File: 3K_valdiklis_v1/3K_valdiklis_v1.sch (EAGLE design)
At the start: 67 parts, among them IC2 L293D, IC4 ATMEGA1284, IC5 DS1307, J4 HEAD3X2, K1 S202T02, K2 S202T02, K3 S202T02, K4 S202T02, K5 S202T02, K6 S202T02, Q4 32.768, T2 TIP120V, X1 Boiler pump, X10 22-23-2031, X11 +12V, X2 Storage tank pump, X3 Radiator pump, X4 4 way valve 1, X5 4 way valve 2, X6 Floor heating, X7 motorized valve 1, X77 PUMP1, X8 motorized valve 2, X9 16MHz, Y1 12mhz

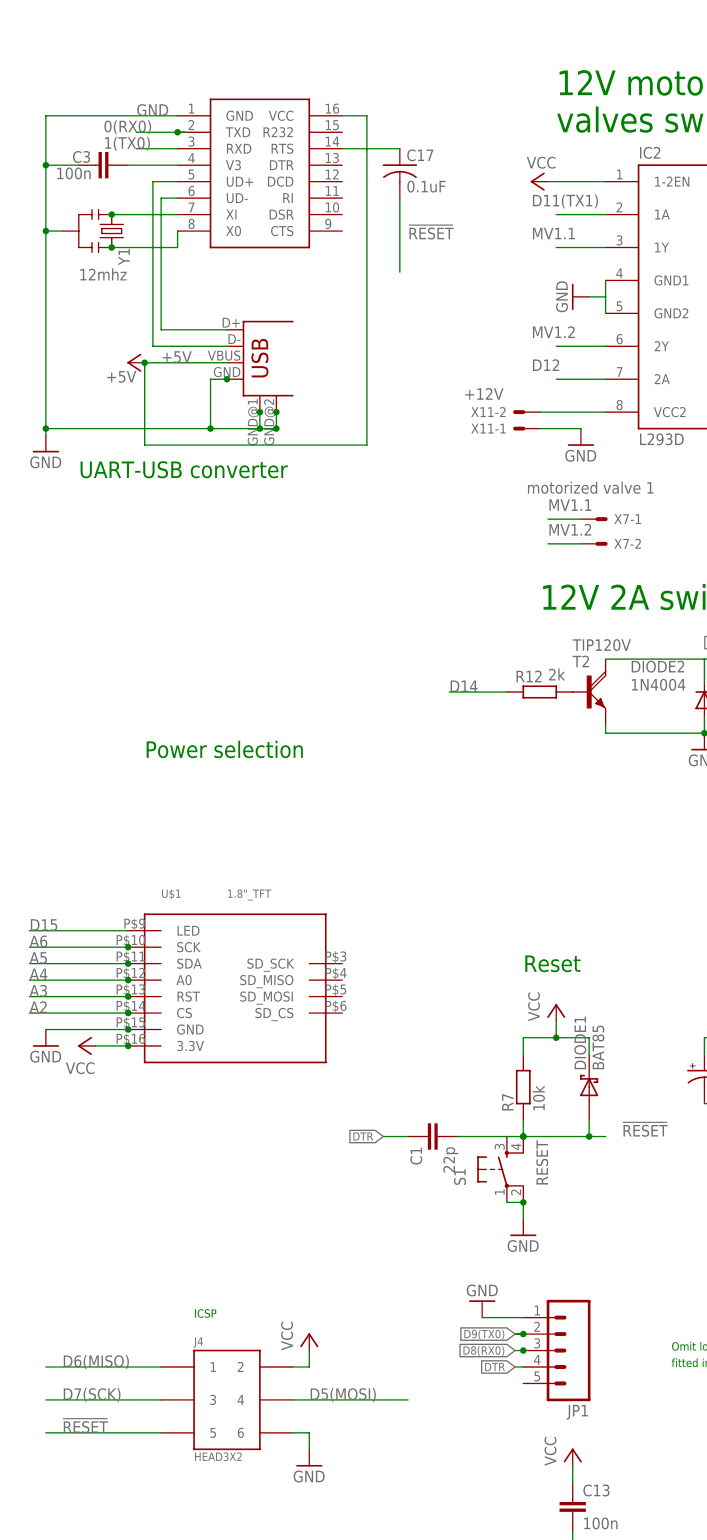
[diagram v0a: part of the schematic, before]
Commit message: trasavimas
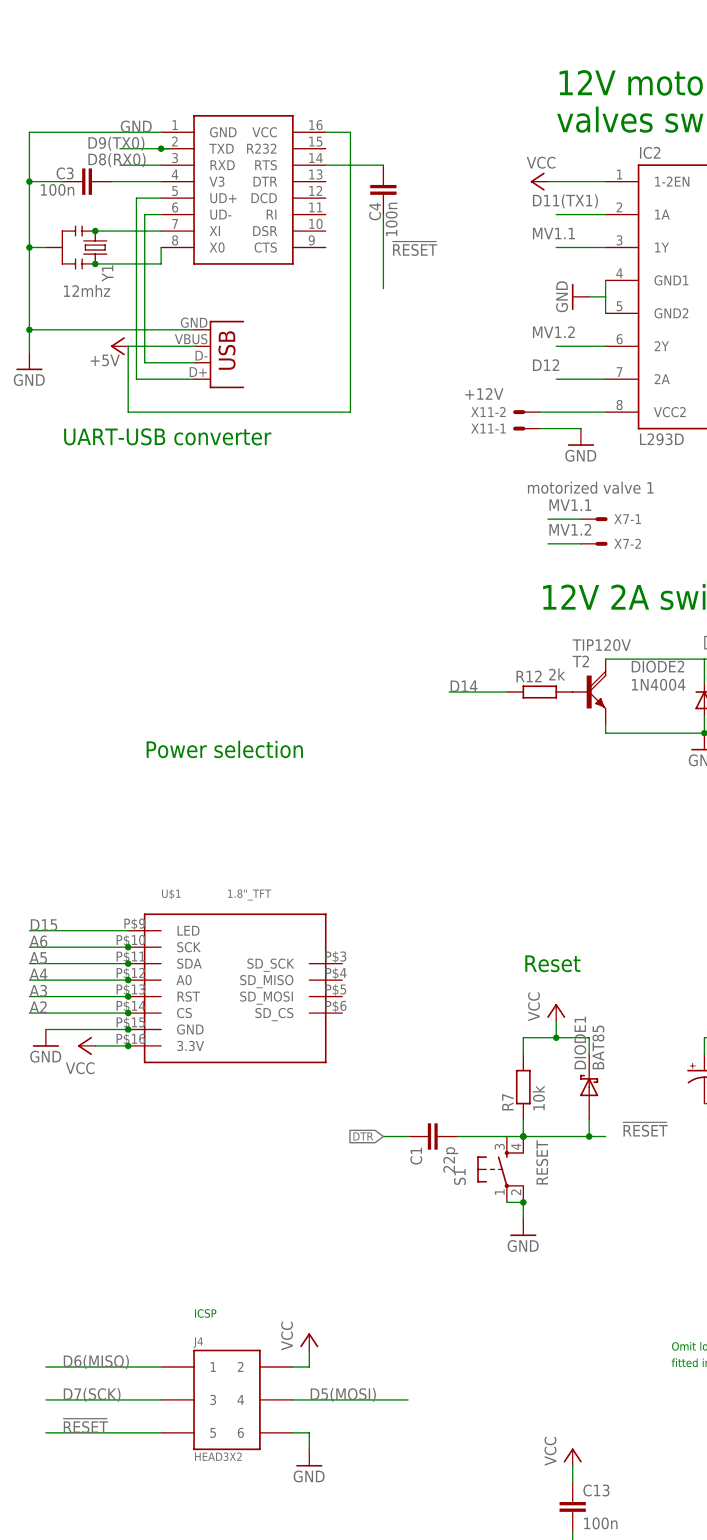
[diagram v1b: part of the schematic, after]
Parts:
- removed C17: 0.1uF, rcl:C-USC0805K
- removed JP1: (no value), SparkFun-Connectors-1:M05PTH
- removed USB1: USB-B-H, con-usb-2:USB-B-H
- added C4: 100n, SparkFun:CAPPTH
- added JP3: USB-B, SparkFun-Connectors-1:USBPTH
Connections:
- removed net 0(RX0): U$2.TXD
- removed net 1(TX0): U$2.RXD
- net !RESET: now also C4.1; no longer C17.2
- net +5V: now also JP3.VBUS; no longer USB1.VBUS
- net D8(RX0): now also U$2.RXD; no longer JP1.3
- net D9(TX0): now also U$2.TXD; no longer JP1.2
- net DTR: no longer JP1.4
- net GND: now also JP3.GND; no longer JP1.1, USB1.GND, USB1.GND@1, USB1.GND@2
- net N$11: now also C4.2; no longer C17.1
- net N$12: now also JP3.D-; no longer USB1.D+
- net N$22: now also JP3.D+; no longer USB1.D-
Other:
- moved on the sheet: C3, Y1
